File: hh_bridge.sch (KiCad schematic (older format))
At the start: 15 parts, among them U8 IRS2304 || U3115S

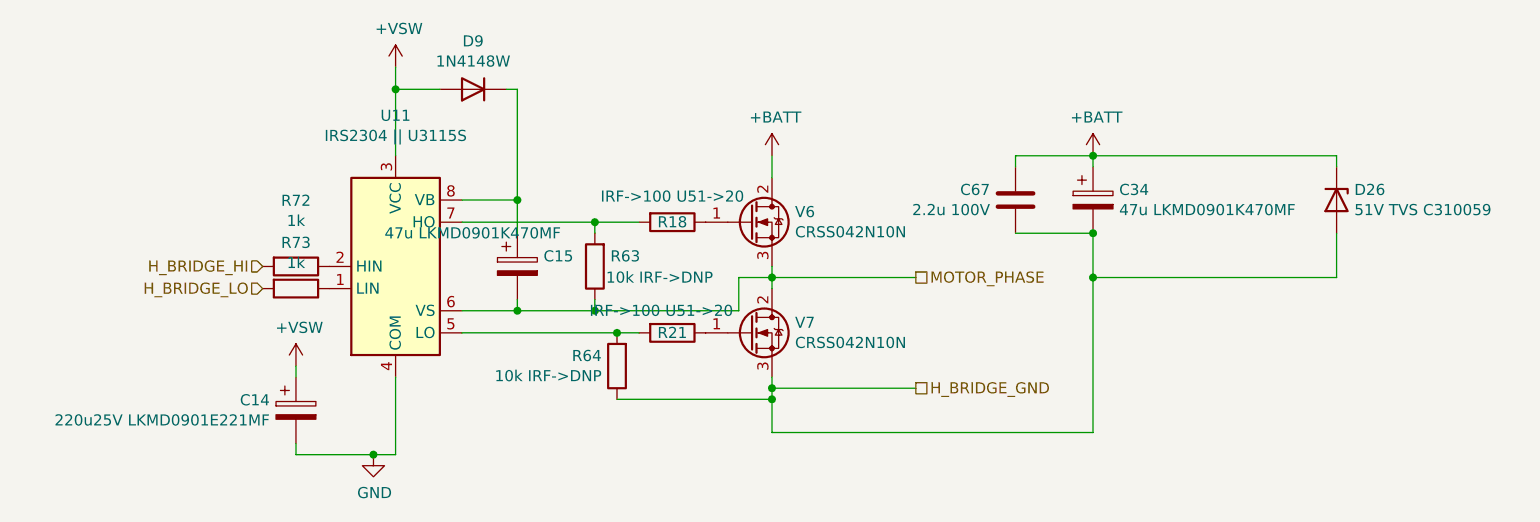
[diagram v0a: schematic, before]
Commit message: prepare production files
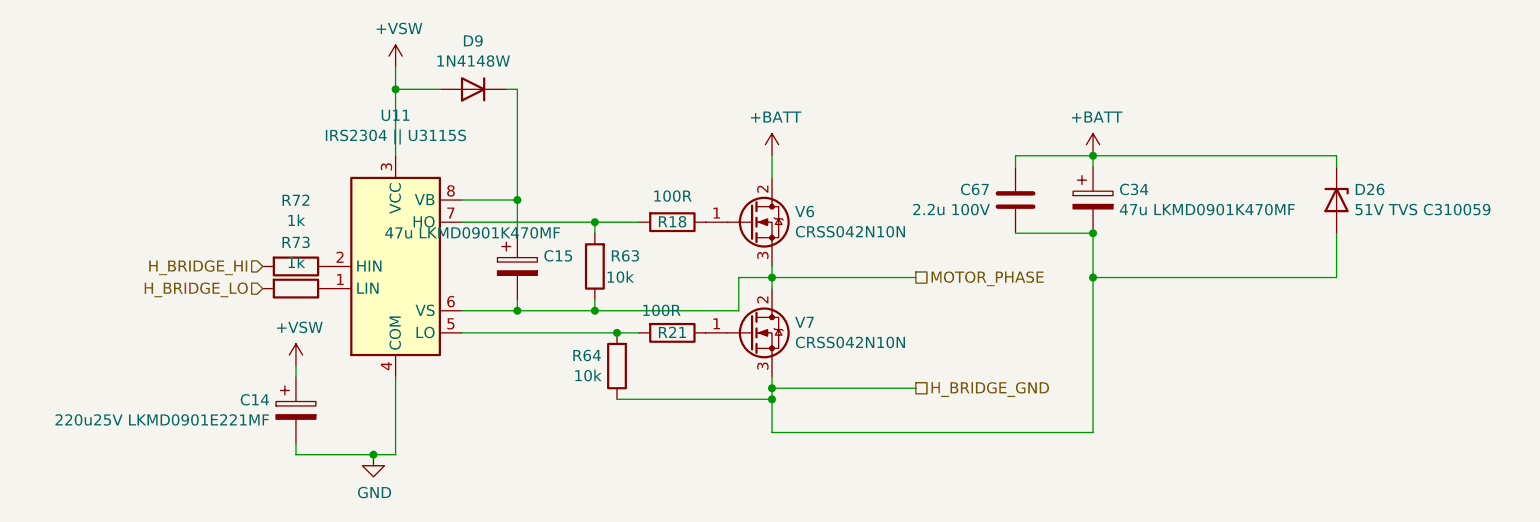
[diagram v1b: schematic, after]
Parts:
- R10, R13: value IRF->100 U51->20 -> 100R
- R50, R51: value 10k IRF->DNP -> 10k
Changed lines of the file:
@@
 AR Path="/5F7A4E71/5F72B1D2" Ref="R34"  Part="1"
 F 0 "R21" V 5200 3600 50  0000 C CNN
-F 1 "IRF->100 U51->20" V 5100 3550 50  0000 C CNN
+F 1 "100R" V 5100 3550 50  0000 C CNN
 F 2 "Resistor_SMD:R_1206_3216Metric" V 5130 3600 50  0001 C CNN
 F 3 "~" H 5200 3600 50  0001 C CNN
@@
 AR Path="/5F7A4E71/5F7824C8" Ref="R33"  Part="1"
 F 0 "R18" V 5200 3100 50  0000 C CNN
-F 1 "IRF->100 U51->20" V 5084 3100 50  0000 C CNN
+F 1 "100R" V 5084 3100 50  0000 C CNN
 F 2 "Resistor_SMD:R_1206_3216Metric" V 5130 3100 50  0001 C CNN
 F 3 "~" H 5200 3100 50  0001 C CNN
@@
 AR Path="/5F7A4E71/5F76BFEE" Ref="R70"  Part="1"
 F 0 "R64" H 5019 3704 50  0000 L CNN
-F 1 "10k IRF->DNP" H 5019 3795 50  0000 L CNN
+F 1 "10k" H 5019 3795 50  0000 L CNN
 F 2 "Resistor_SMD:R_1206_3216Metric" V 4880 3750 50  0001 C CNN
 F 3 "~" H 4950 3750 50  0001 C CNN
@@
 AR Path="/5F7A4E71/5F76CC5E" Ref="R69"  Part="1"
 F 0 "R63" H 4780 3254 50  0000 R CNN
-F 1 "10k IRF->DNP" H 4800 3350 50  0000 R CNN
+F 1 "10k" H 4800 3350 50  0000 R CNN
 F 2 "Resistor_SMD:R_1206_3216Metric" V 4780 3300 50  0001 C CNN
 F 3 "~" H 4850 3300 50  0001 C CNN
